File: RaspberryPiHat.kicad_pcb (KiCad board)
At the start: 2 copper layers, 27.9 x 19.3 mm, 9 parts, among them J1 Raspberry_Pi_2_3, SW1 SW_DPST, U1 DHT22

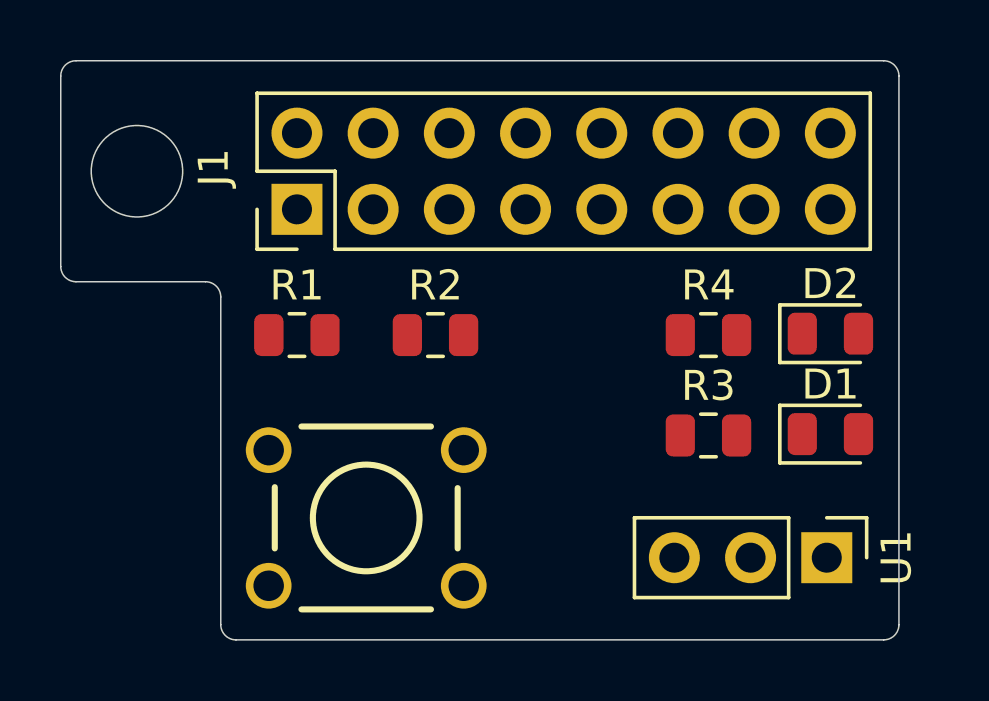
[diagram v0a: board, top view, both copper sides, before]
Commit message: Updated files
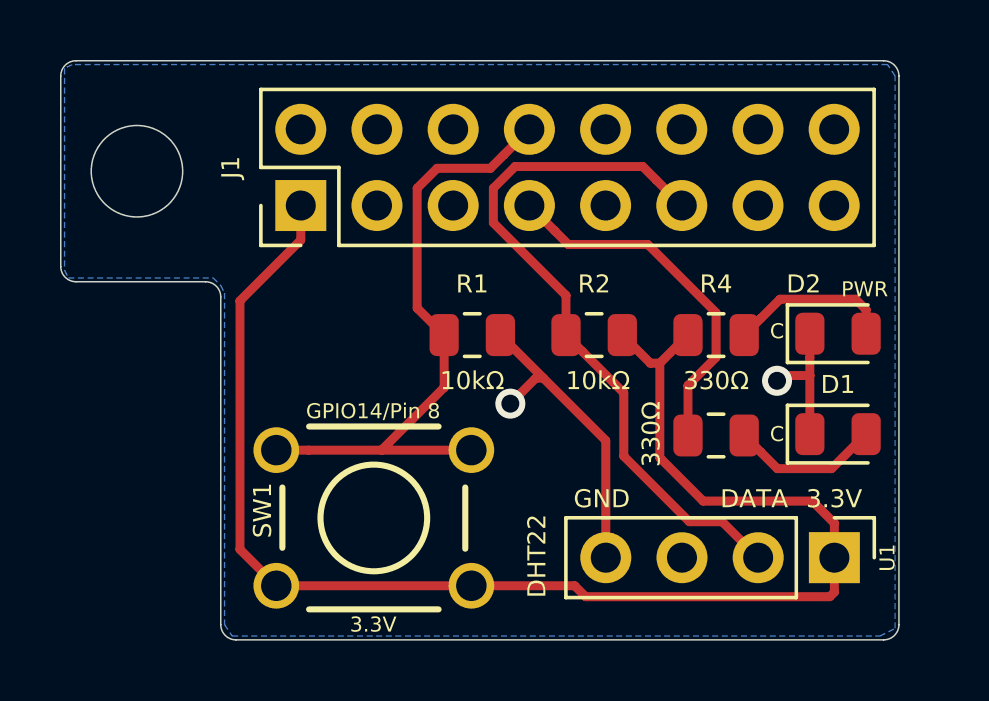
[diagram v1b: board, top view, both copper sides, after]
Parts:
- added G***: LOGO, KiCad Graphics:3HitComboLogoInverted, B.Cu at (95.9, 72.5)
- added REF**: OSHW-Logo_5.7x6mm_SilkScreen, Symbol:OSHW-Logo_5.7x6mm_SilkScreen, B.Cu at (95.0, 77.5)
- R1, R2: value R -> 10kΩ
- R3, R4: value R -> 330Ω
- U1: footprint Connector_PinHeader_2.54mm:PinHeader_1x03_P2.54mm_Vertical -> Connector_PinHeader_2.54mm:PinHeader_1x04_P2.54mm_Vertical
- moved R1 5.84 mm to (98.3, 72.9)
- moved R2 5.29 mm to (102.4, 72.9)
- moved R3 0.25 mm to (106.4, 76.2)
- moved R4 0.25 mm to (106.4, 72.9)
- moved U1 0.25 mm to (110.4, 80.3)
- moved D1 0.25 mm to (110.5, 76.2)
- moved D2 0.25 mm to (110.5, 72.9)
- moved SW1 0.25 mm to (95.0, 79.0), turned to 180 degrees
- moved J1 0.18 mm to (92.6, 68.6)
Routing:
- net /3v3: track 0.00 -> 48.0 mm
- net Net-(J1-Pad11): track 0.00 -> 23.7 mm
- net /button_input: track 0.00 -> 21.0 mm
- net GND: track 0.00 -> 14.8 mm, vias 0 -> 2
- net Net-(J1-Pad7): track 0.00 -> 12.2 mm
- net Net-(D2-Pad2): track 0.00 -> 5.50 mm
- net Net-(D1-Pad2): track 0.00 -> 5.00 mm
- added copper zone on B.Cu, net GND
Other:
- board text added: "3.3V"
- board text added: "Button: GPIO14 LED: GPIO4"
- board text added: "C"
- board text added: "DATA"
- board text added: "GND"
- board text added: "GPIO14/Pin 8"
- board text added: "PWR"
- board text added: "Raspberry Pi Full Stack Hat Ver 1.0"
